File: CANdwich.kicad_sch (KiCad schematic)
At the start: 48 parts, among them J3 DE9_Receptacle, J4 Conn_01x04_Socket, J5 USB_C_Receptacle_USB2.0, U1 AP2127K-3.3, U2 STM32F072CBT6, U3 SN6505BDBV, U4 AP2204K-5.0TRG1, U6 ISO1050DUB, Y1 16MHz

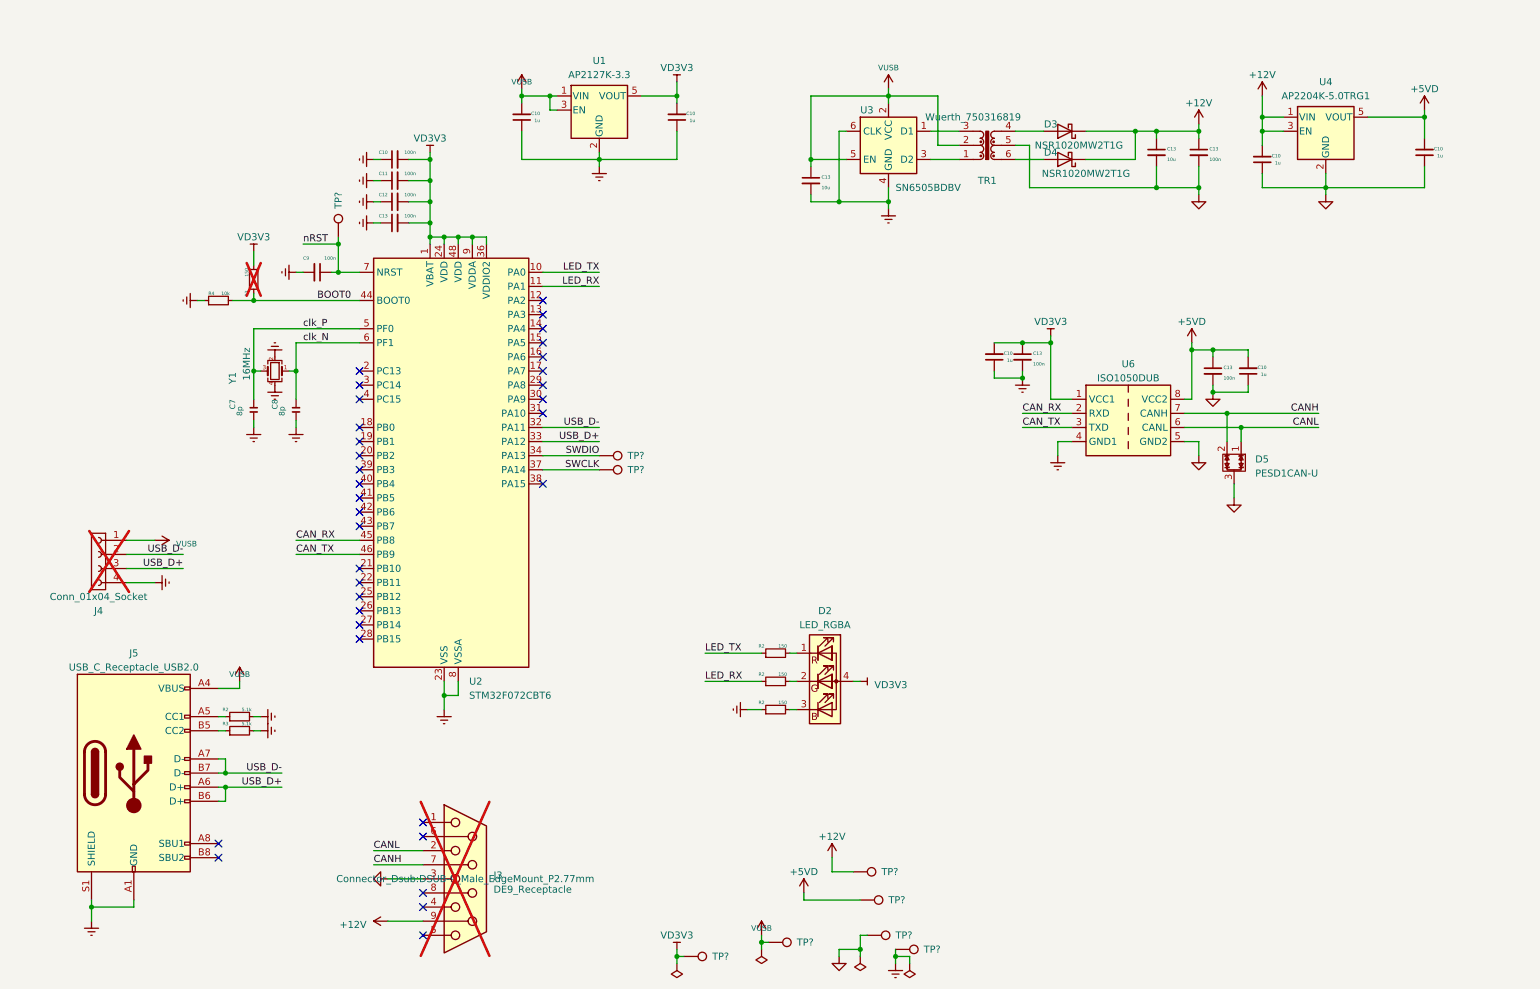
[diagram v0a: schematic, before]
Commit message: V1.0 Generate external enclosure
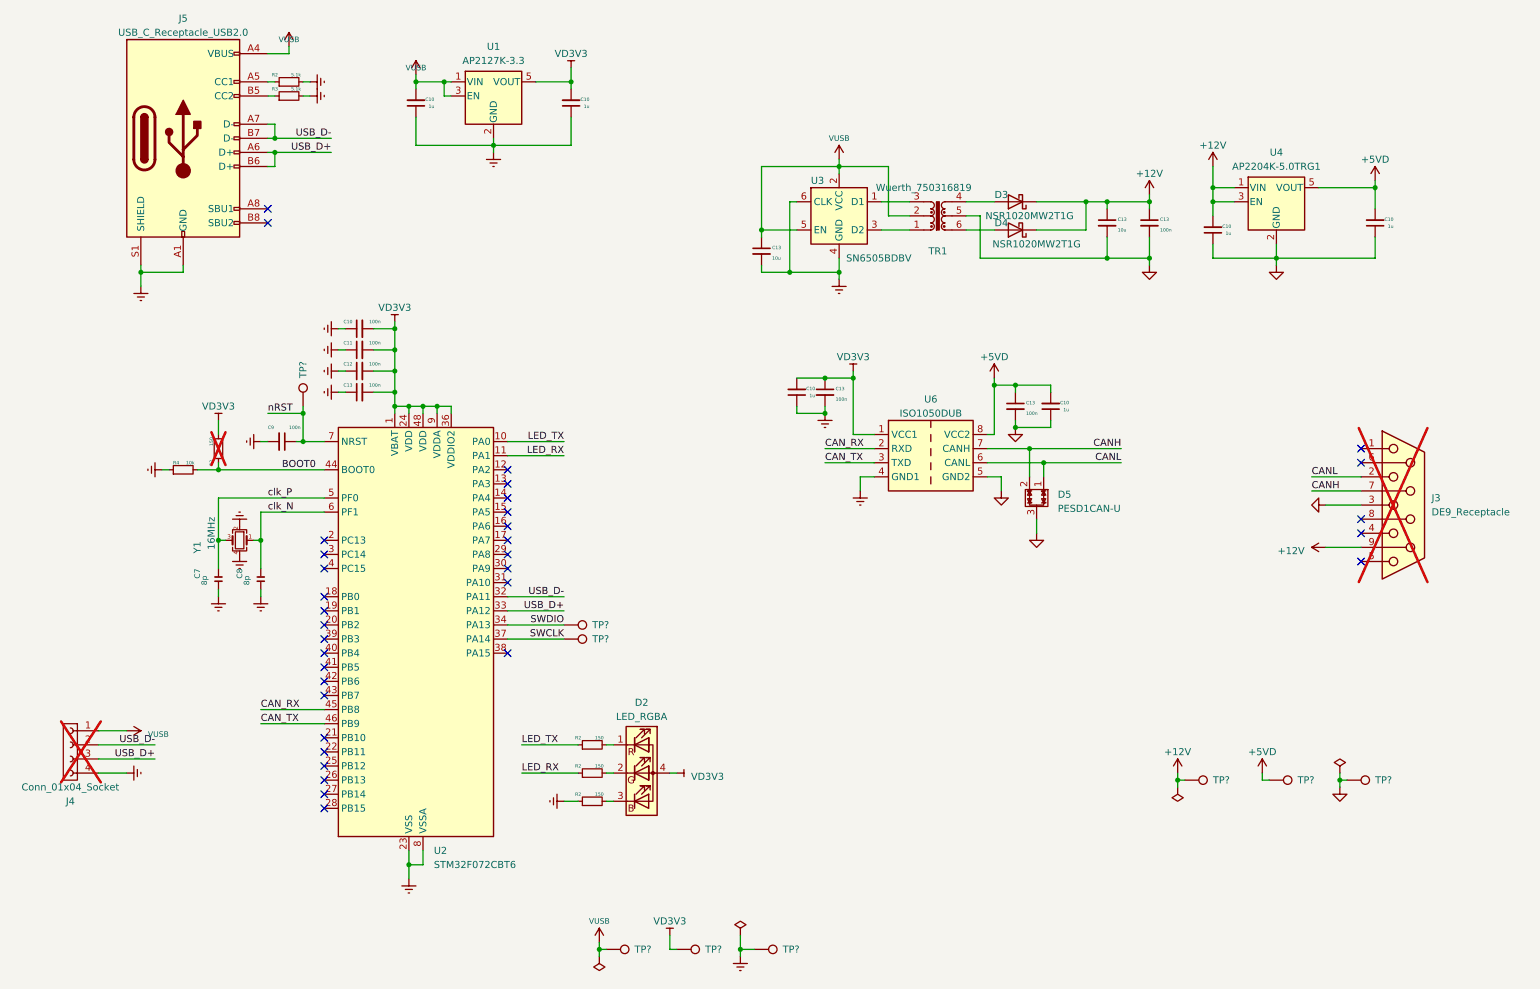
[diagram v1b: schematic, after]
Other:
- title: (none) -> CANdwich
- moved on the sheet: C10, C11, C12, C13, C7, C8, C9, D2, D3, D4, D5, J3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
